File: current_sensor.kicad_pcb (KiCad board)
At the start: 2 copper layers, 13.7 x 10.7 mm, 3 parts, among them J3 Conn_01x03_Male, U1 ACS781xLRTR-100B

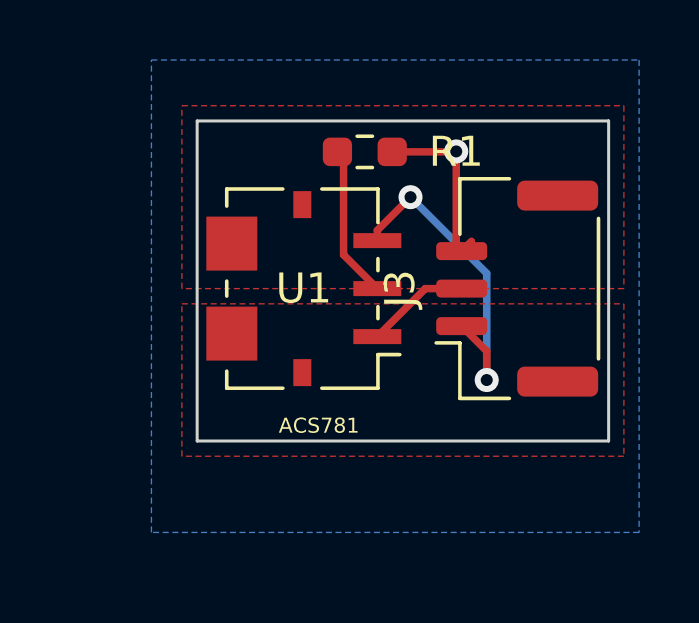
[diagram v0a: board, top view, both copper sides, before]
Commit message: make it smaller
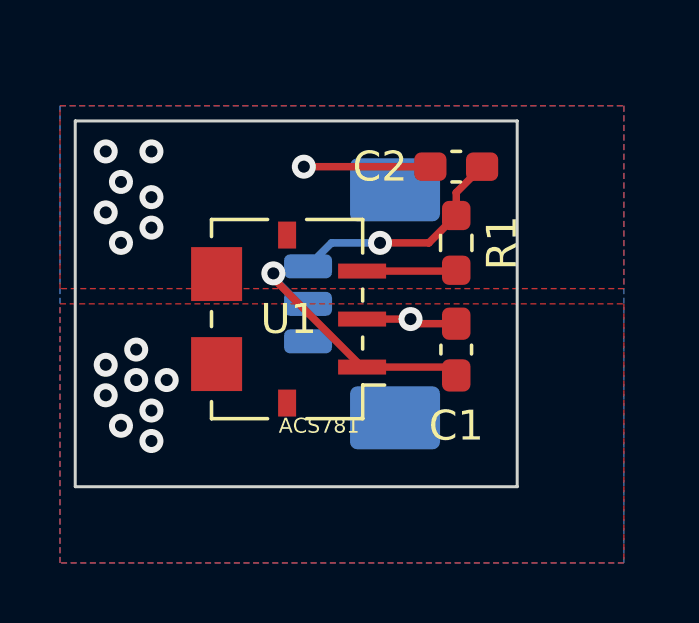
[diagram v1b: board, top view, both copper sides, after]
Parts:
- added C1: 0.1 uF, Capacitor_SMD:C_0603_1608Metric_Pad1.08x0.95mm_HandSolder, F.Cu at (212.9, 89.9)
- added C2: Cf, Capacitor_SMD:C_0603_1608Metric_Pad1.08x0.95mm_HandSolder, F.Cu at (212.9, 83.8)
- J3: footprint Connector_Molex:Molex_CLIK-Mate_502386-0370_1x03-1MP_P1.25mm_Horizontal -> Connector_Molex:Molex_PicoBlade_53261-0371_1x03-1MP_P1.25mm_Horizontal; moved to B.Cu
- R1: value R -> Rf
- moved J3 4.60 mm to (210.3, 88.4), turned to -90 degrees
- moved R1 4.30 mm to (212.9, 86.4), turned to 90 degrees
- moved U1 1.14 mm to (207.3, 88.9)
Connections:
- J3 pad 3: GND -> GNDREF
- R1 pad 1: GND -> Net-(U1-Pad3)
- R1 pad 2: Net-(R1-Pad2) -> Net-(J3-Pad1)
- U1 pad 2: Net-(R1-Pad2) -> GNDREF
- U1 pad 3: Net-(J3-Pad1) -> Net-(U1-Pad3)
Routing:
- net GNDREF: track 0.00 -> 7.42 mm, vias 0 -> 2
- net GND: track 6.00 -> 0.00 mm, vias 1 -> 0
- net +3.3V: track 3.47 -> 9.27 mm, vias 0 -> 1
- net Net-(R1-Pad2): track 5.24 -> 0.00 mm
- net Net-(J3-Pad1): track 11.2 -> 7.63 mm, vias 2 -> 1
- net Net-(U1-Pad3): track 0.00 -> 3.15 mm
- net -12V: vias 0 -> 8
- net +12V: vias 0 -> 7
- added copper zone on B.Cu, net GNDREF
- removed copper zone on B.Cu, net GND
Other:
- board size 13.7 x 10.7 mm -> 14.7 x 12.2 mm
